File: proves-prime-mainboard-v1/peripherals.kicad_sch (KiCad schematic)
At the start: 38 parts, among them IC3 RV-3028-C7_32.768kHz_1ppm_TA_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, J6 Breakout, J7 Breakout, J8 Molex 503398-1892, U3 MCP25625-E/ML, U4 AP3602AKTR-G1, U5 LSM6DSOTR, U6 LSM303AGRTR, Y2 16MHZ 12 pf

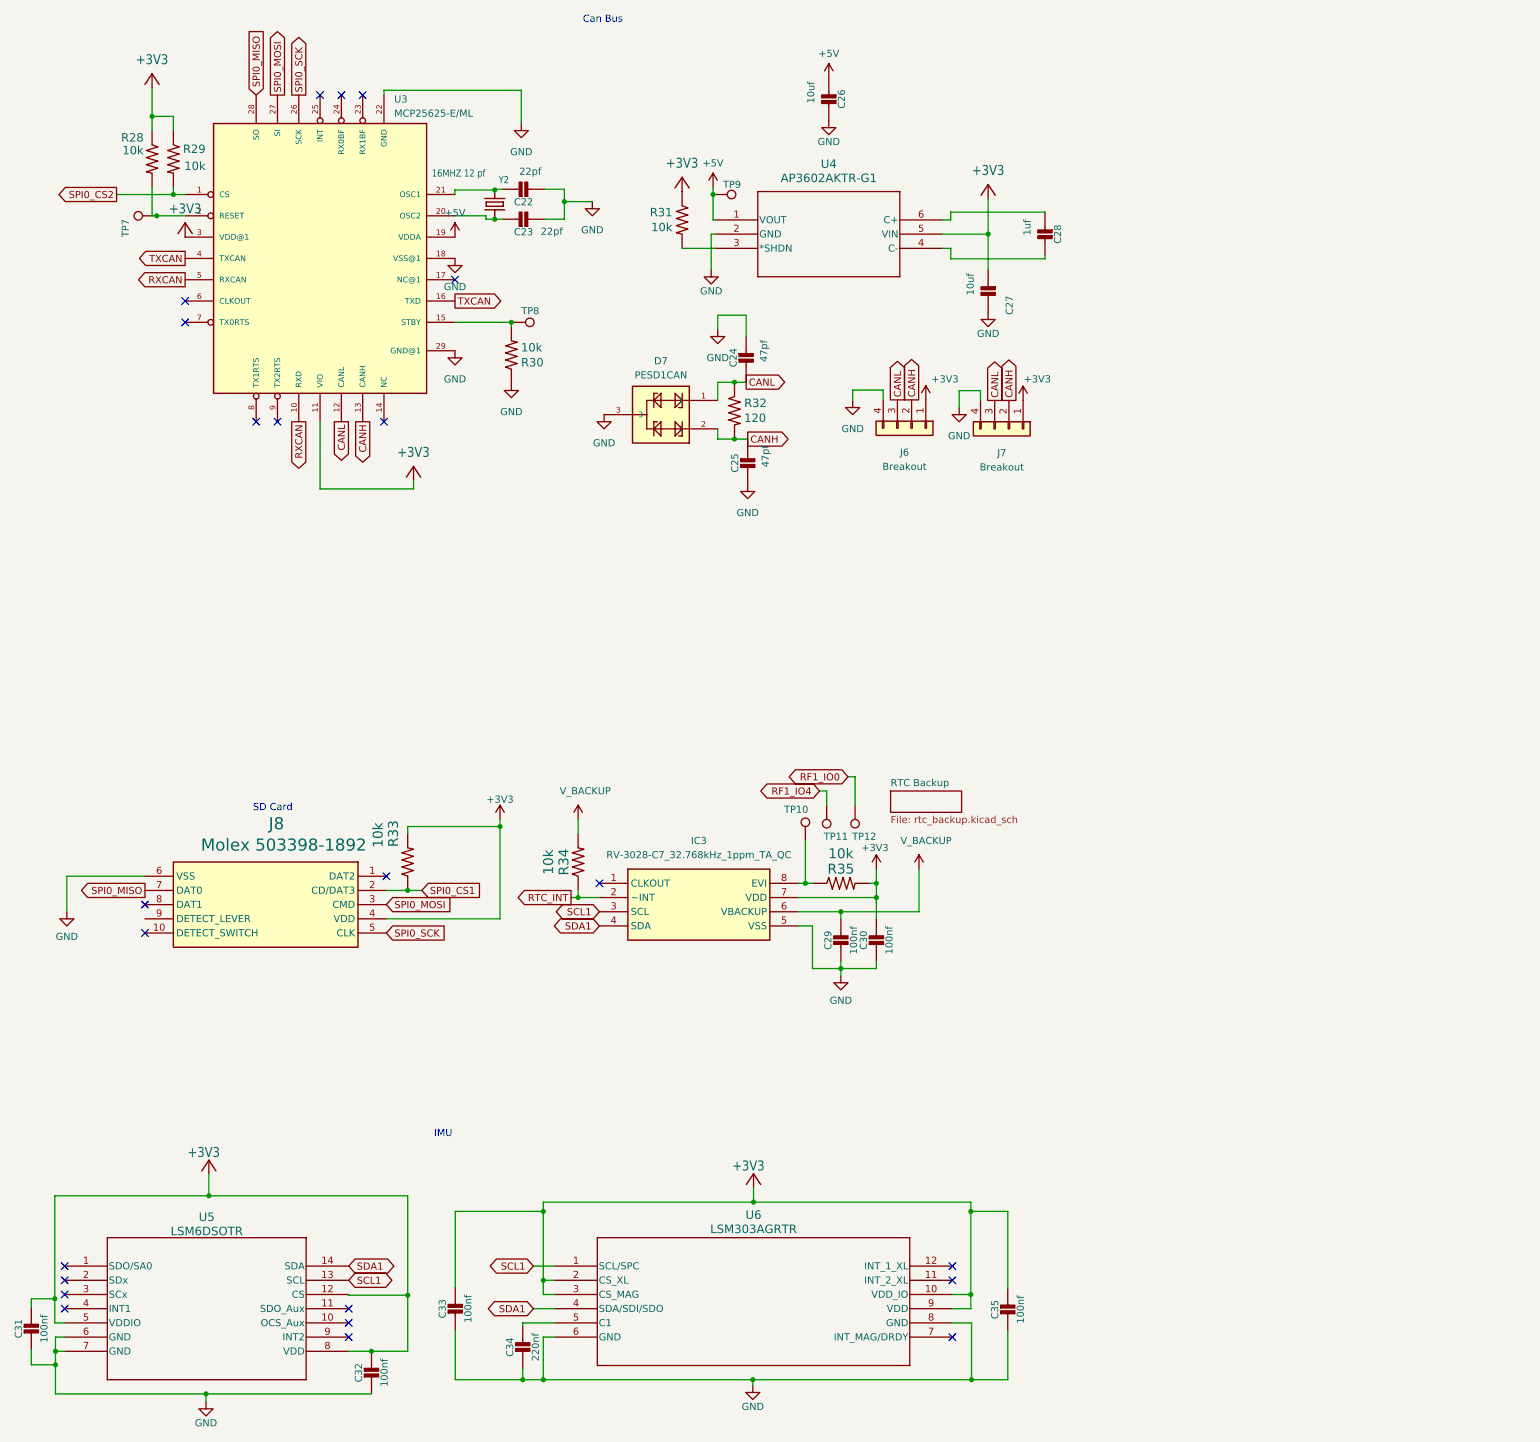
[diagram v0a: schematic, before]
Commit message: Migrated Temperature Sensor
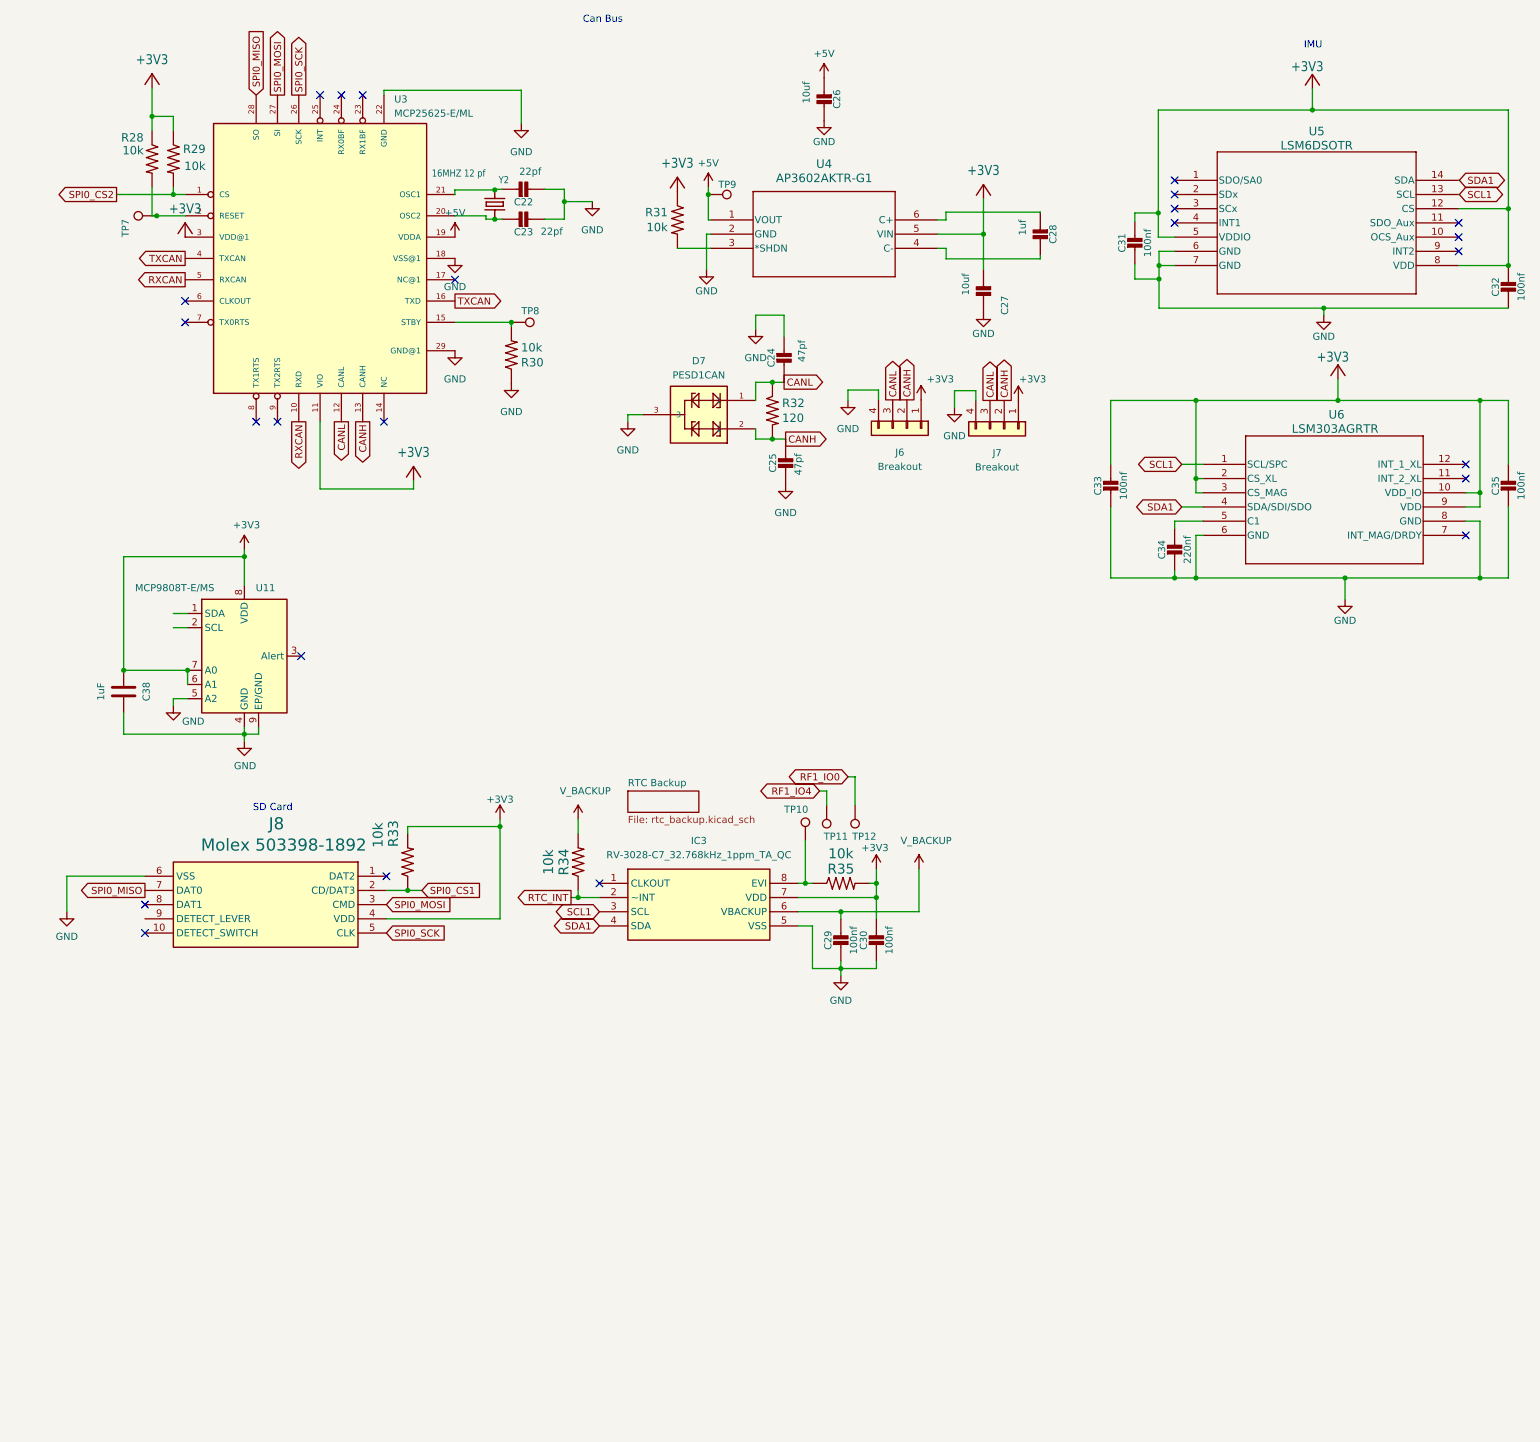
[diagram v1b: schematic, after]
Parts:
- added C38: 1uF, Capacitor_SMD:C_0805_2012Metric, symbol Device:C
- added U11: MCP9808T-E/MS, Package_SO:MSOP-8-1EP_3x3mm_P0.65mm_EP1.5x1.8mm_ThermalVias, symbol Sensor_Temperature:MCP9808_DFN
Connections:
- net +3V3: now also C38.1, U11.6 (A1), U11.7 (A0), U11.8 (VDD)
- net GND: now also C38.2, U11.4 (GND), U11.5 (A2), U11.9 (EP/GND)
- no-connect marks 23 -> 24
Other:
- moved on the sheet: C24, C25, C26, C27, C28, C31, C32, C33, C34, C35, D7, J6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
